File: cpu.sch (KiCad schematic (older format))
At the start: 26 parts, among them U1 68000D, U10 74LS244, U11 74LS373, U12 74LS244, U13 74LS373, U2 FAT_AGNUS_8375, U33 74LS258, U37 74LS32, U5 GARY_5719, X1 XTAL

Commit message: Almost all components positioned
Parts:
- E666: footprint (none) -> Raemixx500:C_Axial_L6.3mm_D2.5mm_P10.16mm
- FB101, FB102: footprint (none) -> Raemixx500:EMI_Filter_Long
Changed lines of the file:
@@
 F 0 "FB102" V 9220 10260 50  0000 C CNN
 F 1 "150" V 9310 10260 50  0000 C CNN
-F 2 "" V 9240 10260 50  0001 C CNN
+F 2 "Raemixx500:EMI_Filter_Long" V 9240 10260 50  0001 C CNN
 F 3 "~" H 9310 10260 50  0001 C CNN
 	1    9310 10260
@@
 F 0 "E666" H 9692 10516 50  0000 L CNN
 F 1 "22p" H 9692 10425 50  0000 L CNN
-F 2 "" H 9600 10470 50  0001 C CNN
+F 2 "Raemixx500:C_Axial_L6.3mm_D2.5mm_P10.16mm" H 9600 10470 50  0001 C CNN
 F 3 "~" H 9600 10470 50  0001 C CNN
 	1    9600 10470
@@
 F 0 "FB101" V 7800 10160 50  0000 C CNN
 F 1 "68" V 7890 10160 50  0000 C CNN
-F 2 "" V 7820 10160 50  0001 C CNN
+F 2 "Raemixx500:EMI_Filter_Long" V 7820 10160 50  0001 C CNN
 F 3 "~" H 7890 10160 50  0001 C CNN
 	1    7890 10160

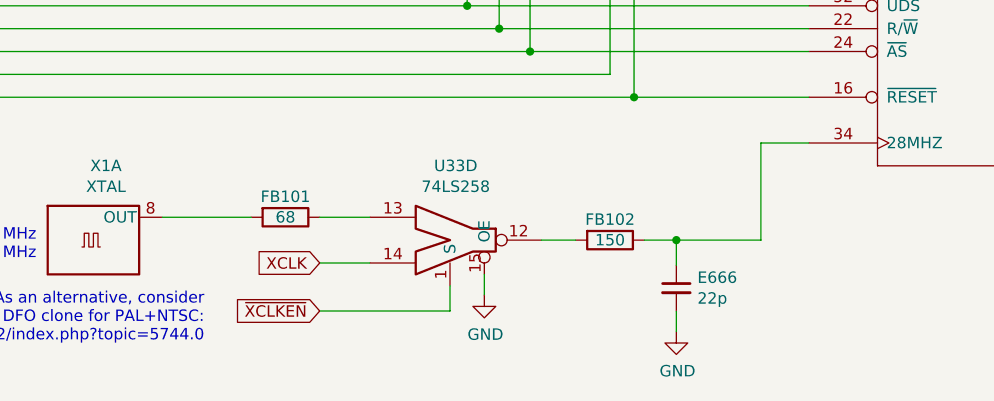
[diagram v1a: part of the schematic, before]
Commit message: Work in progress
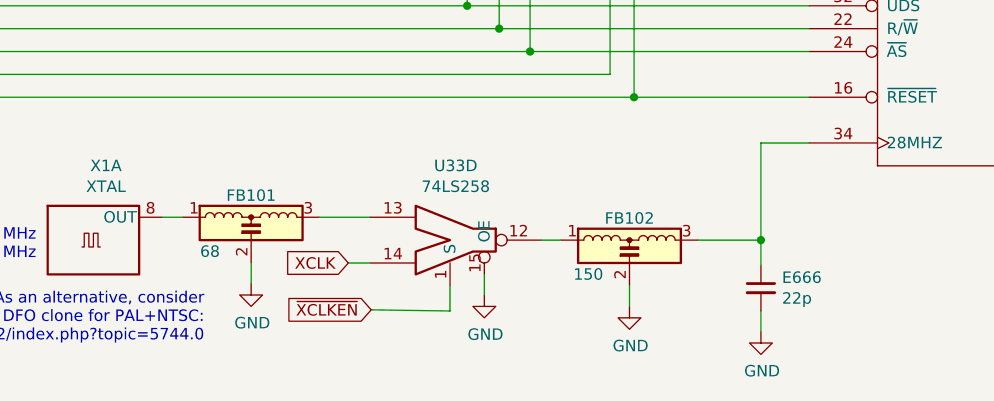
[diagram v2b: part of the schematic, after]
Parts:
- removed FB101: 68, Raemixx500:EMI_Filter_Long, symbol Device:R
- removed FB102: 150, Raemixx500:EMI_Filter_Long, symbol Device:R
- added FB101: 68, Raemixx500:EMI_Filter_Long, symbol Device:EMI_Filter_LCL
- added FB102: 150, Raemixx500:EMI_Filter_Long, symbol Device:EMI_Filter_LCL
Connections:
- net GND: now also FB101.2, FB102.2
- net at E666.1, U2.34 (28MHZ): now also FB102.3
- net at U33.12: now also FB102.1
- net at U33.13: now also FB101.3
- net at X1.8 (OUT): now also FB101.1
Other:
- moved on the sheet: E666
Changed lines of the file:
@@
 $EndComp
 Wire Wire Line
-	9010 10260 9160 10260
-$Comp
-L Device:R FB102
-U 1 1 5CC23FBE
-P 9310 10260
-F 0 "FB102" V 9220 10260 50  0000 C CNN
-F 1 "150" V 9310 10260 50  0000 C CNN
-F 2 "Raemixx500:EMI_Filter_Long" V 9240 10260 50  0001 C CNN
-F 3 "~" H 9310 10260 50  0001 C CNN
-	1    9310 10260
-	0    1    1    0
-$EndComp
-Wire Wire Line
-	9460 10260 9600 10260
+	9010 10260 9095 10260
 $Comp
 L Device:C_Small E666
 U 1 1 5CC5EA40
-P 9600 10470
-F 0 "E666" H 9692 10516 50  0000 L CNN
-F 1 "22p" H 9692 10425 50  0000 L CNN
-F 2 "Raemixx500:C_Axial_L6.3mm_D2.5mm_P10.16mm" H 9600 10470 50  0001 C CNN
-F 3 "~" H 9600 10470 50  0001 C CNN
-	1    9600 10470
+P 9970 10470
+F 0 "E666" H 10062 10516 50  0000 L CNN
+F 1 "22p" H 10062 10425 50  0000 L CNN
+F 2 "Raemixx500:C_Axial_L6.3mm_D2.5mm_P10.16mm" H 9970 10470 50  0001 C CNN
+F 3 "~" H 9970 10470 50  0001 C CNN
+	1    9970 10470
 	1    0    0    -1
 $EndComp
 Wire Wire Line
-	9600 10370 9600 10260
-Connection ~ 9600 10260
+	9970 10370 9970 10260
 Wire Wire Line
-	9600 10570 9600 10660
+	9970 10570 9970 10660
 $Comp
 L power:GND #PWR0200
 U 1 1 5CD0F28E
-P 9600 10660
-F 0 "#PWR0200" H 9600 10410 50  0001 C CNN
-F 1 "GND" H 9605 10487 50  0000 C CNN
-F 2 "" H 9600 10660 50  0001 C CNN
-F 3 "" H 9600 10660 50  0001 C CNN
-	1    9600 10660
+P 9970 10660
+F 0 "#PWR0200" H 9970 10410 50  0001 C CNN
+F 1 "GND" H 9975 10487 50  0000 C CNN
+F 2 "" H 9970 10660 50  0001 C CNN
+F 3 "" H 9970 10660 50  0001 C CNN
+	1    9970 10660
 	1    0    0    -1
 $EndComp
 Wire Wire Line
-	8260 10360 8040 10360
-Text GLabel 8040 10360 0    50   Input ~ 0
+	8260 10360 8165 10360
+Text GLabel 8165 10360 0    50   Input ~ 0
 XCLK
 Wire Wire Line
 	8260 10160 8040 10160
-$Comp
-L Device:R FB101
-U 1 1 5CD85D7B
-P 7890 10160
-F 0 "FB101" V 7800 10160 50  0000 C CNN
-F 1 "68" V 7890 10160 50  0000 C CNN
-F 2 "Raemixx500:EMI_Filter_Long" V 7820 10160 50  0001 C CNN
-F 3 "~" H 7890 10160 50  0001 C CNN
-	1    7890 10160
-	0    1    1    0
-$EndComp
-Text GLabel 8040 10570 0    50   Input ~ 0
+Text GLabel 8265 10565 0    50   Input ~ 0
 ~XCLKEN
 Wire Wire Line
 	8610 10570 8610 10460
 Wire Wire Line
-	8040 10570 8610 10570
+	8265 10565 8610 10570
 Wire Wire Line
 	8760 10410 8760 10500
@@
 $EndComp
 Wire Wire Line
-	7350 10160 7740 10160
+	7350 10160 7440 10160
 $Comp
 L xtal:XTAL X1
@@
 Wire Wire Line
 	9970 9835 10180 9835
-Wire Wire Line
-	9600 10260 9970 10260
 Text Notes 6800 10350 2    50   ~ 0
 PAL: 28.37516 MHz\nNTSC: 28.63636 MHz
+$Comp
+L Device:EMI_Filter_LCL E?
+U 1 1 5D645153
+P 7740 10260
+AR Path="/5D2DC3A1/5D645153" Ref="E?"  Part="1"
+AR Path="/5CAE5331/5D645153" Ref="FB101"  Part="1"
+F 0 "FB101" H 7740 10455 50  0000 C CNN
+F 1 "68" H 7560 10210 50  0000 C CNN
+F 2 "Raemixx500:EMI_Filter_Long" V 7740 10260 50  0001 C CNN
+F 3 "http://www.murata.com/~/media/webrenewal/support/library/catalog/products/emc/emifil/c31e.ashx?la=en-gb" V 7740 10260 50  0001 C CNN
+	1    7740 10260
+	1    0    0    -1
+$EndComp
+Wire Wire Line
+	7740 10360 7740 10450
+$Comp
+L power:GND #PWR0266
+U 1 1 5D73BDA5
+P 7740 10450
+F 0 "#PWR0266" H 7740 10200 50  0001 C CNN
+F 1 "GND" H 7745 10277 50  0000 C CNN
+F 2 "" H 7740 10450 50  0001 C CNN
+F 3 "" H 7740 10450 50  0001 C CNN
+	1    7740 10450
+	1    0    0    -1
+$EndComp
+Connection ~ 9970 10260
+$Comp
+L Device:EMI_Filter_LCL FB?
+U 1 1 5D8302E3
+P 9395 10360
+AR Path="/5D2DC3A1/5D8302E3" Ref="FB?"  Part="1"
+AR Path="/5CAE5331/5D8302E3" Ref="FB102"  Part="1"
+F 0 "FB102" H 9395 10555 50  0000 C CNN
+F 1 "150" H 9215 10310 50  0000 C CNN
+F 2 "Raemixx500:EMI_Filter_Long" V 9395 10360 50  0001 C CNN
+F 3 "http://www.murata.com/~/media/webrenewal/support/library/catalog/products/emc/emifil/c31e.ashx?la=en-gb" V 9395 10360 50  0001 C CNN
+	1    9395 10360
+	1    0    0    -1
+$EndComp
+Wire Wire Line
+	9395 10460 9395 10550
+$Comp
+L power:GND #PWR0267
+U 1 1 5D8302EE
+P 9395 10550
+F 0 "#PWR0267" H 9395 10300 50  0001 C CNN
+F 1 "GND" H 9400 10377 50  0000 C CNN
+F 2 "" H 9395 10550 50  0001 C CNN
+F 3 "" H 9395 10550 50  0001 C CNN
+	1    9395 10550
+	1    0    0    -1
+$EndComp
+Wire Wire Line
+	9695 10260 9970 10260
+Wire Bus Line
+	1370 3735 1370 3935
 Wire Bus Line
 	1370 3235 1370 3435
 Wire Bus Line
-	1370 3735 1370 3935
-Wire Bus Line
 	13405 5535 13405 6235

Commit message: Top layer done!
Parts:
- X1: footprint Oscillator:Oscillator_SMD_TXC_7C-4Pin_5.0x3.2mm -> Raemixx500:Xtal
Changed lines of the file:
@@
 F 0 "X1" H 7105 10585 50  0000 C CNN
 F 1 "XTAL" H 7105 10494 50  0000 C CNN
-F 2 "Oscillator:Oscillator_SMD_TXC_7C-4Pin_5.0x3.2mm" H 7150 9610 50  0001 C CNN
+F 2 "Raemixx500:Xtal" H 7150 9610 50  0001 C CNN
 F 3 "http://www.txccorp.com/download/products/osc/7C_o.pdf" H 6950 10260 50  0001 C CNN
 	1    7050 10260

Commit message: Add C99 on PCB
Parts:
- C99: footprint (none) -> Raemixx500:C_Axial_L6.3mm_D2.5mm_P10.16mm
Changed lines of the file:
@@
 F 0 "C99" H 14590 8661 50  0000 L CNN
 F 1 "100n" H 14590 8570 50  0000 L CNN
-F 2 "" H 14513 8465 50  0001 C CNN
+F 2 "Raemixx500:C_Axial_L6.3mm_D2.5mm_P10.16mm" H 14513 8465 50  0001 C CNN
 F 3 "~" H 14475 8615 50  0001 C CNN
 	1    14475 8615

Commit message: Use KiCad footprint for oscillator
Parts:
- X1: footprint Raemixx500:Xtal -> Oscillator:Oscillator_DIP-14
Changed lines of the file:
@@
 F 0 "X1" H 7105 10585 50  0000 C CNN
 F 1 "XTAL" H 7105 10494 50  0000 C CNN
-F 2 "Raemixx500:Xtal" H 7150 9610 50  0001 C CNN
+F 2 "Oscillator:Oscillator_DIP-14" H 7150 9610 50  0001 C CNN
 F 3 "http://www.txccorp.com/download/products/osc/7C_o.pdf" H 6950 10260 50  0001 C CNN
 	1    7050 10260
